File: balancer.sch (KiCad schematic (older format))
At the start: 7 parts, among them IC1 TLV3404, J1 S4B-XH-SM4-TB, J2 CONN_01X01, J3 CONN_01X01, Q1 IRF7455PBF

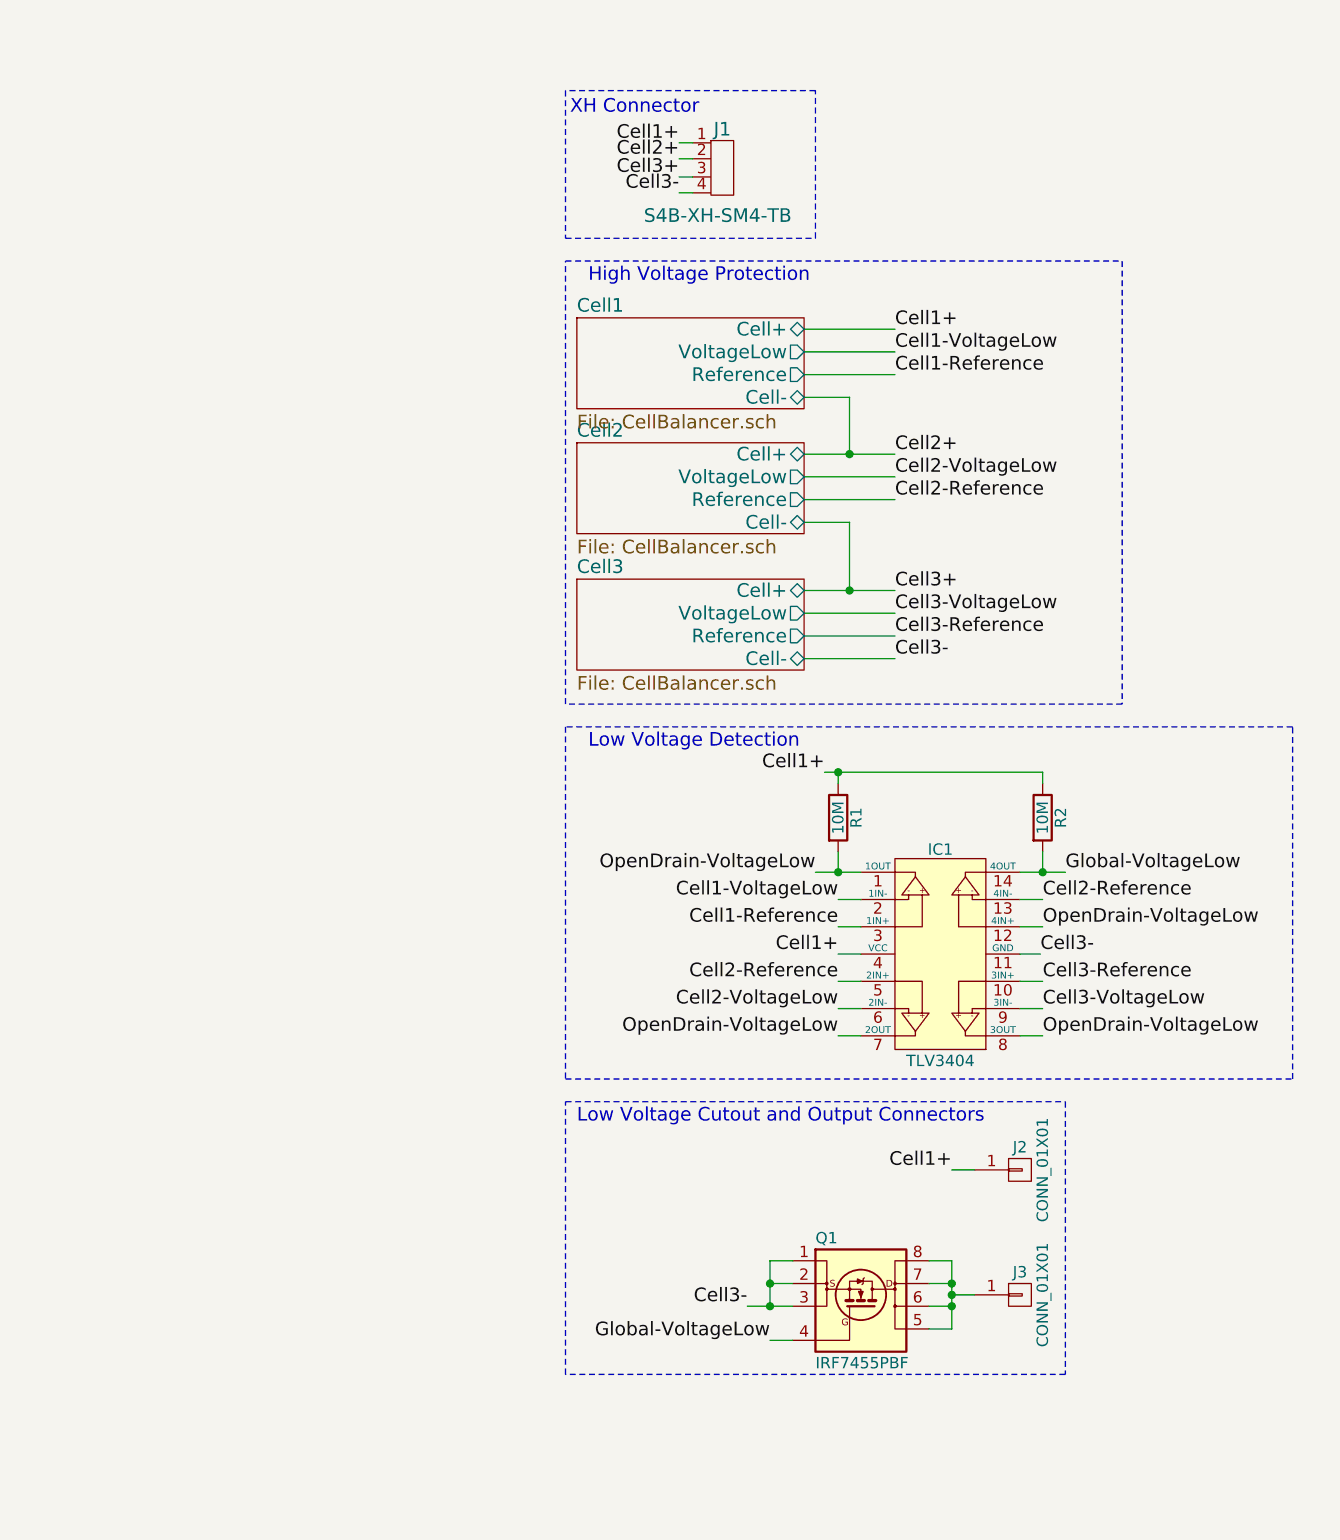
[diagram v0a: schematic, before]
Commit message: layout finalized
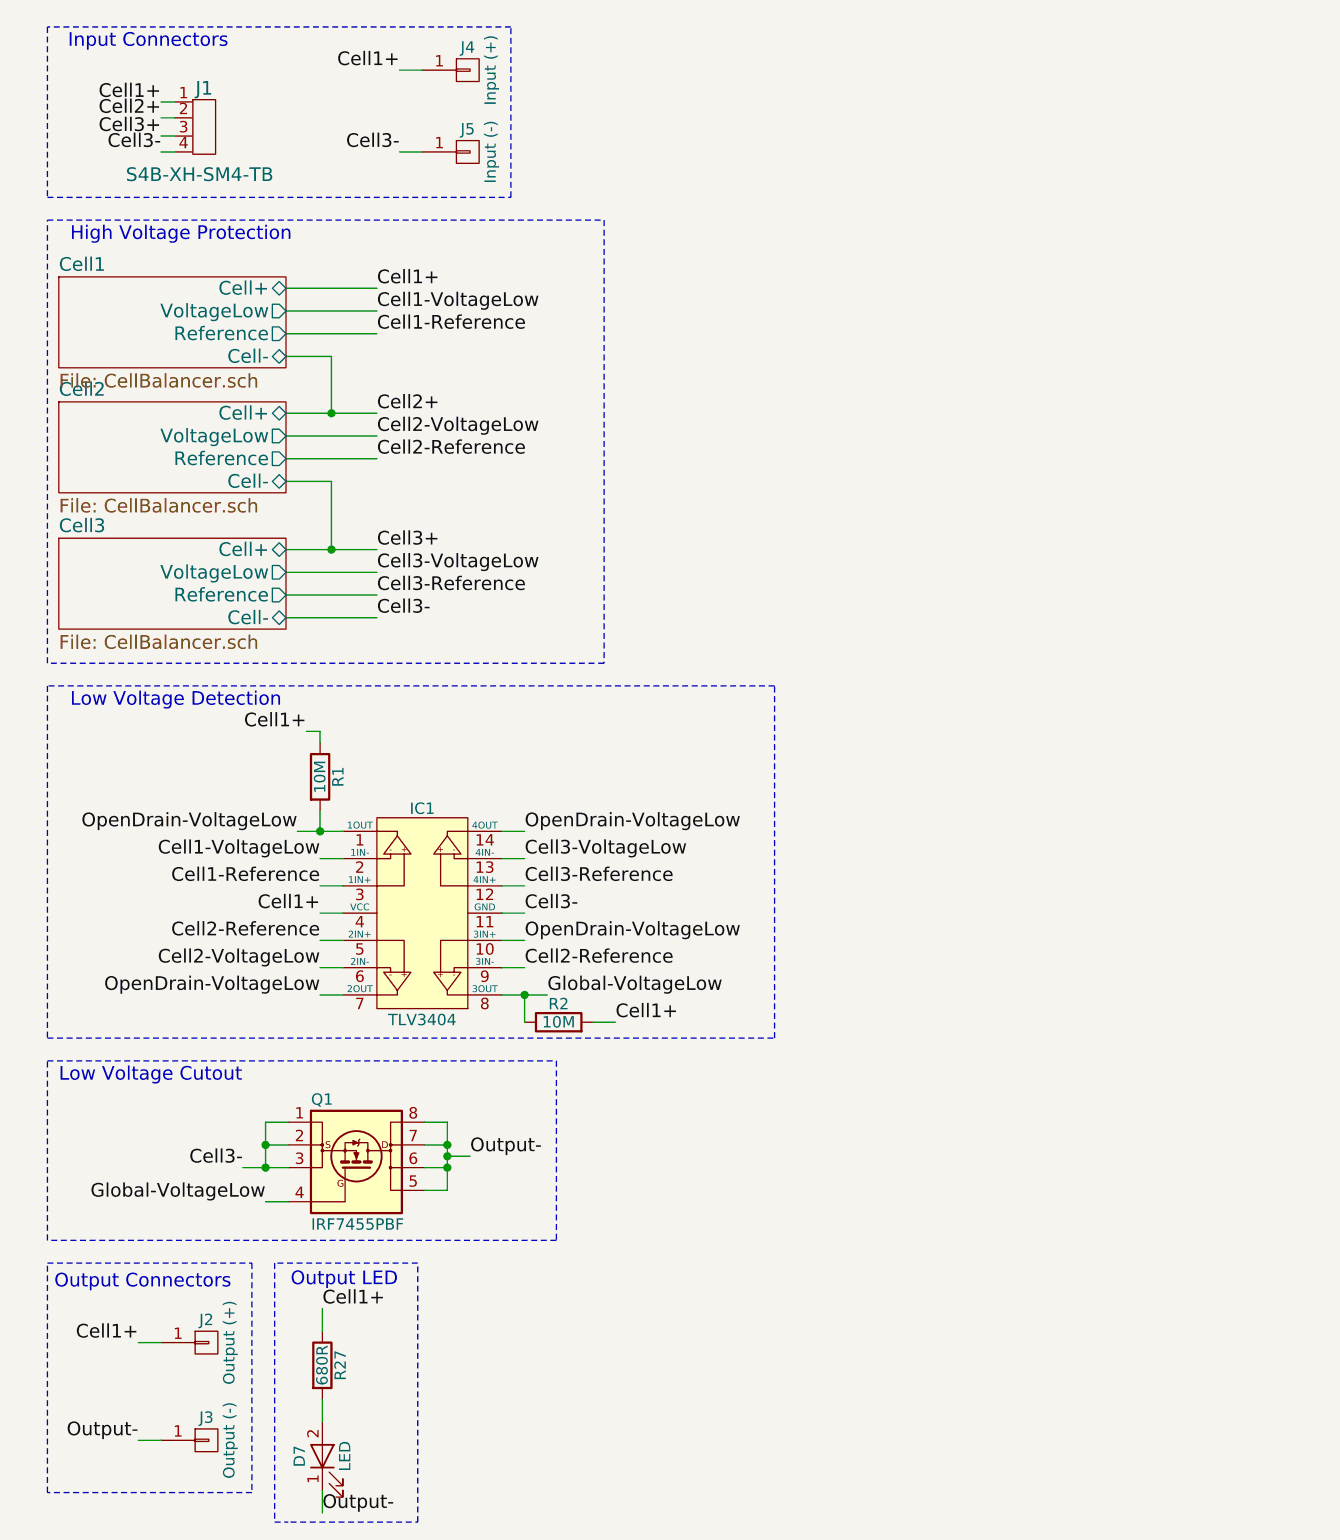
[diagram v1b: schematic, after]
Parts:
- added D7: LED, LEDs:LED_0805, symbol LED
- added J4: Input (+), balancer:Solder_Terminal_4x4mm, symbol CONN_01X01
- added J5: Input (-), balancer:Solder_Terminal_4x4mm, symbol CONN_01X01
- added R27: 680R, Resistors_SMD:R_0805, symbol R
- J2: value CONN_01X01 -> Output (+); footprint Pin_Headers:Pin_Header_Straight_1x01_Pitch2.54mm -> balancer:Solder_Terminal_4x4mm
- J3: value CONN_01X01 -> Output (-); footprint Pin_Headers:Pin_Header_Straight_1x01_Pitch2.54mm -> balancer:Solder_Terminal_4x4mm
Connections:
- net Cell1+: now also R2.2, J4.1 (P1), R27.1; no longer R2.1
- net Cell2-Reference: now also IC1.9 (3IN-); no longer IC1.13 (4IN-)
- net Cell3-: now also J5.1 (P1)
- net Cell3-Reference: now also IC1.12 (4IN+); no longer IC1.10 (3IN+)
- net Cell3-VoltageLow: now also IC1.13 (4IN-); no longer IC1.9 (3IN-)
- net Global-VoltageLow: now also IC1.8 (3OUT), R2.1; no longer IC1.14 (4OUT), R2.2
- net OpenDrain-VoltageLow: now also IC1.10 (3IN+), IC1.14 (4OUT); no longer IC1.12 (4IN+), IC1.8 (3OUT)
- net Output-: now reaches J3.1 (P1), Q1.5 (D), Q1.6 (D), Q1.7 (D), Q1.8 (D)
- net Output-: now also D7.1 (K)
- new net: D7.2 (A), R27.2
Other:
- note added: "Input Connectors"
- note added: "Low Voltage Cutout"
- note added: "Output Connectors"
- note added: "Output LED"
- note removed: "Low Voltage Cutout and Output Connectors"
- note removed: "XH Connector"
- moved on the sheet: IC1, J1, J2, J3, Q1, R1, R2
